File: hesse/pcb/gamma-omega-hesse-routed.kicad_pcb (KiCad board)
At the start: 2 copper layers, 232.8 x 111.4 mm, 47 parts

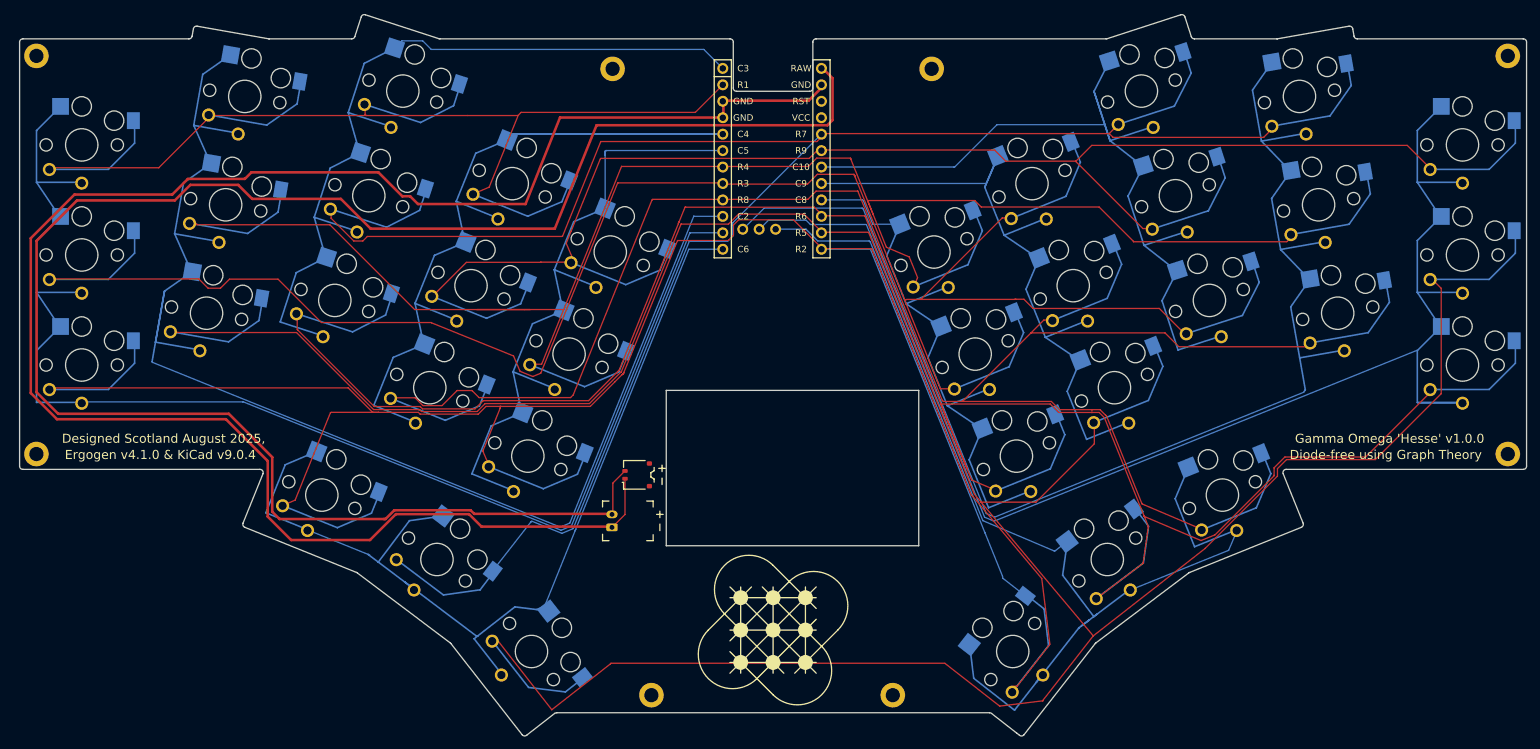
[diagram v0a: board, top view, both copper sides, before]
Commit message: clean
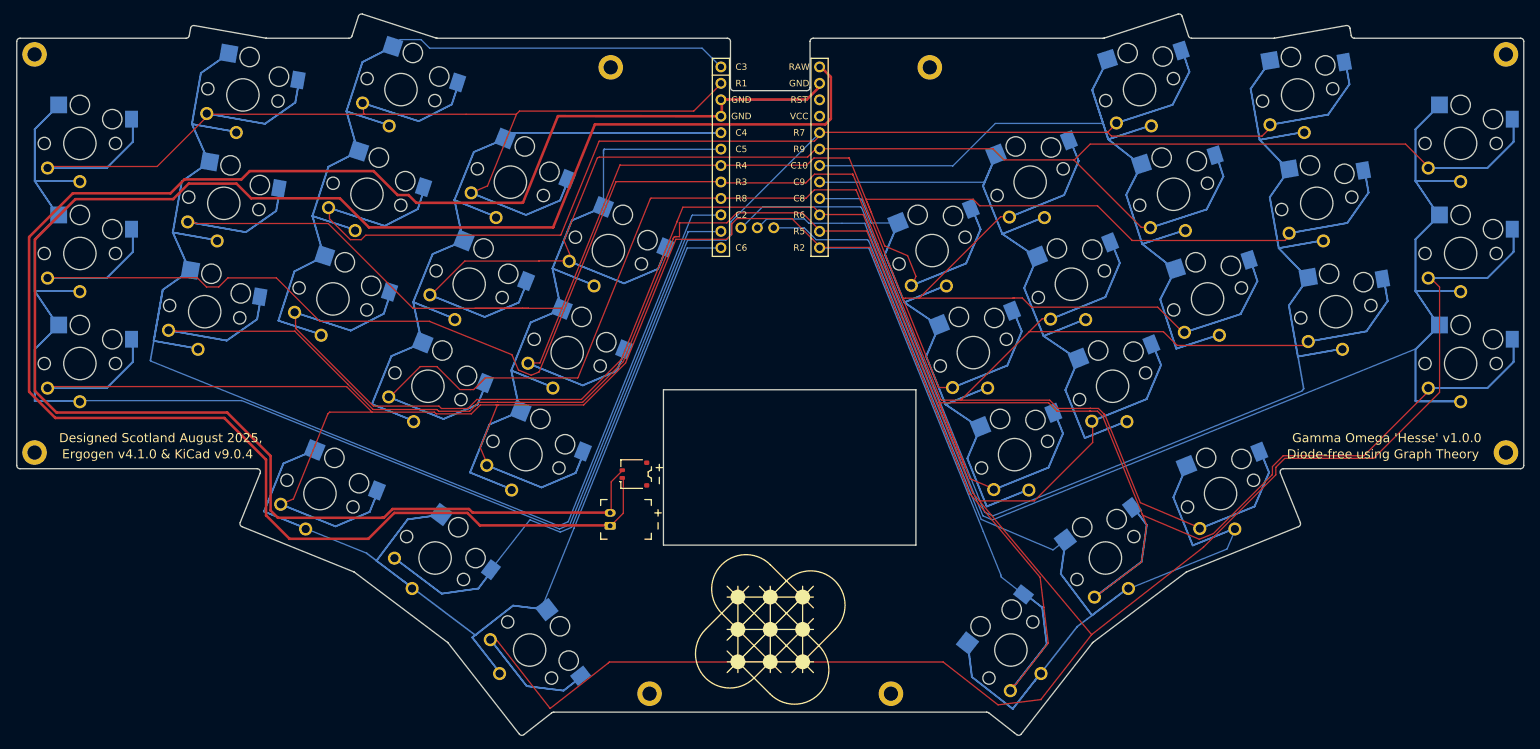
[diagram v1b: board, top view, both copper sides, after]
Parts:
- moved CONN1 0.43 mm to (135.2, 117.2)
- moved S24 0.37 mm to (237.6, 58.7)
- moved S4 0.37 mm to (68.8, 92.2)
- moved S6 0.37 mm to (74.7, 58.7)
- moved S12 0.37 mm to (116.0, 72.2)
- moved S31 0.37 mm to (193.9, 114.2)
- moved S10 0.37 mm to (103.3, 103.7)
- moved H6 0.37 mm to (180.8, 54.4)
- moved S8 0.37 mm to (93.9, 74.0)
- moved S9 0.37 mm to (99.1, 57.9)
- moved S15 0.37 mm to (131.2, 82.7)
- moved S5 0.37 mm to (71.7, 75.4)
- moved S23 0.37 mm to (240.6, 75.4)
- moved JST1 0.37 mm to (131.4, 124.2)
- moved S21 0.37 mm to (262.8, 66.2)
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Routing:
- net R5: track 495.9 -> 569.3 mm
- net R7: track 328.3 -> 401.3 mm
- net R1: track 198.1 -> 271.0 mm
- net R4: track 308.9 -> 381.7 mm
- net R9: track 259.0 -> 331.8 mm
- net R3: track 327.5 -> 400.2 mm
- net C1: track 205.6 -> 278.1 mm
- net C4: track 161.9 -> 234.3 mm
- net C3: track 124.0 -> 196.4 mm
- net C9: track 102.8 -> 175.2 mm
- net C5: track 100.3 -> 172.7 mm
- net C8: track 87.0 -> 159.4 mm
- net C12: track 217.6 -> 289.9 mm
- net C11: track 201.5 -> 273.8 mm
- net C10: track 126.9 -> 199.3 mm
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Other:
- outline, holes or cut-outs redrawn

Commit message: shift
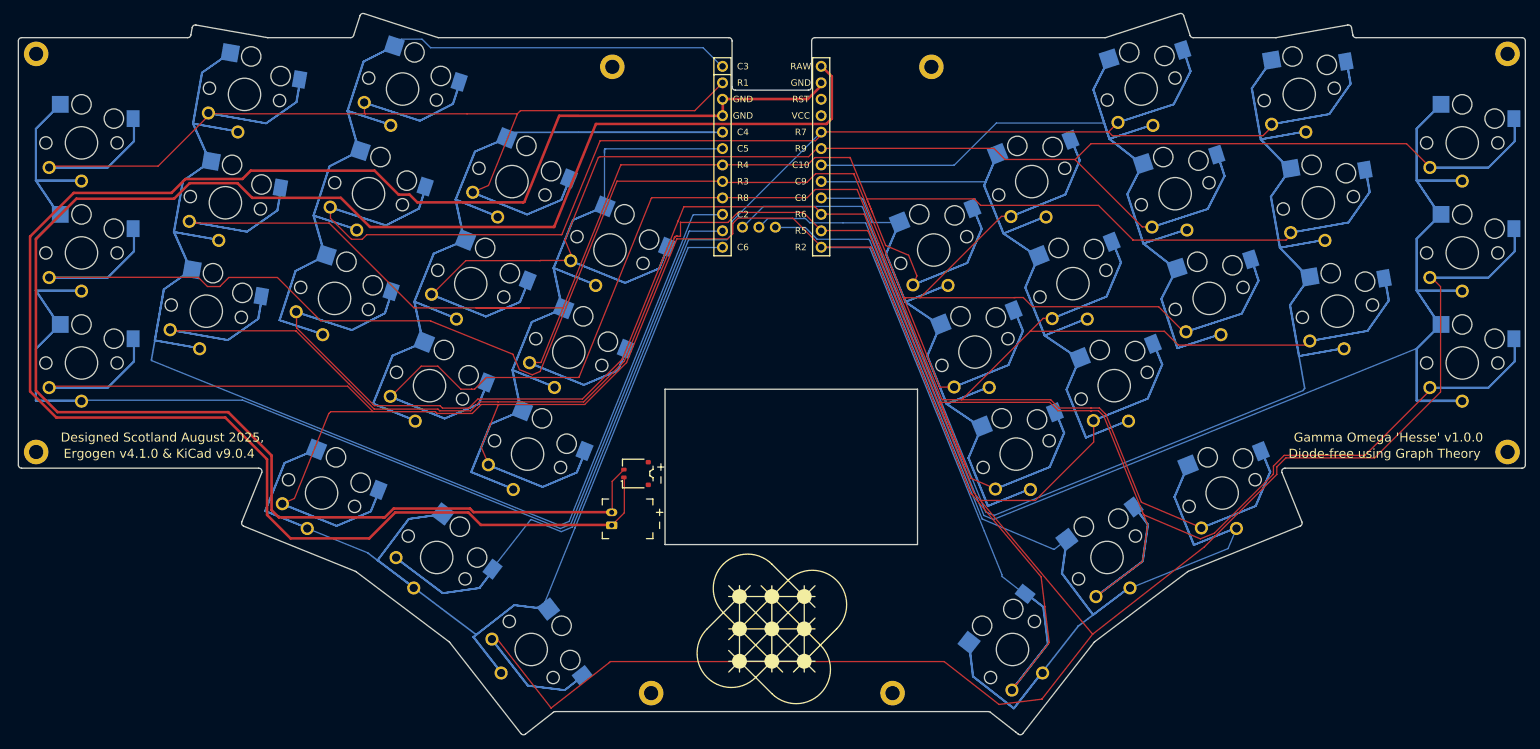
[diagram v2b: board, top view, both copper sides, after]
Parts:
- moved S14 0.26 mm to (125.0, 98.4)
- moved S5 0.26 mm to (72.0, 75.3)
- moved S2 0.26 mm to (49.8, 83.1)
- moved S12 0.26 mm to (116.3, 72.1)
- moved JST1 0.26 mm to (131.7, 124.2)
- moved S7 0.26 mm to (88.8, 90.1)
- moved S35 0.26 mm to (208.2, 130.1)
- moved S25 0.26 mm to (223.9, 90.1)
- moved H6 0.26 mm to (181.0, 54.3)
- moved H3 0.26 mm to (42.8, 113.8)
- moved S15 0.26 mm to (131.4, 82.6)
- moved S1 0.26 mm to (49.8, 100.1)
- moved H1 0.26 mm to (42.8, 52.3)
- moved S11 0.26 mm to (109.9, 87.8)
- moved S33 0.26 mm to (181.4, 82.6)
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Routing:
- net R7: track 401.3 -> 474.2 mm
- net R9: track 331.8 -> 404.8 mm
- net R3: track 400.2 -> 473.1 mm
- net R1: track 271.0 -> 343.9 mm
- net R8: track 390.5 -> 463.4 mm
- net R6: track 435.9 -> 508.8 mm
- net R2: track 471.0 -> 543.9 mm
- net R5: track 569.3 -> 642.2 mm
- net R4: track 381.7 -> 454.6 mm
- net C12: track 289.9 -> 362.3 mm
- net C9: track 175.2 -> 247.6 mm
- net C5: track 172.7 -> 245.0 mm
- net C1: track 278.1 -> 350.4 mm
- net C8: track 159.4 -> 231.8 mm
- net C2: track 281.1 -> 353.4 mm
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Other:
- outline, holes or cut-outs redrawn

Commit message: clean
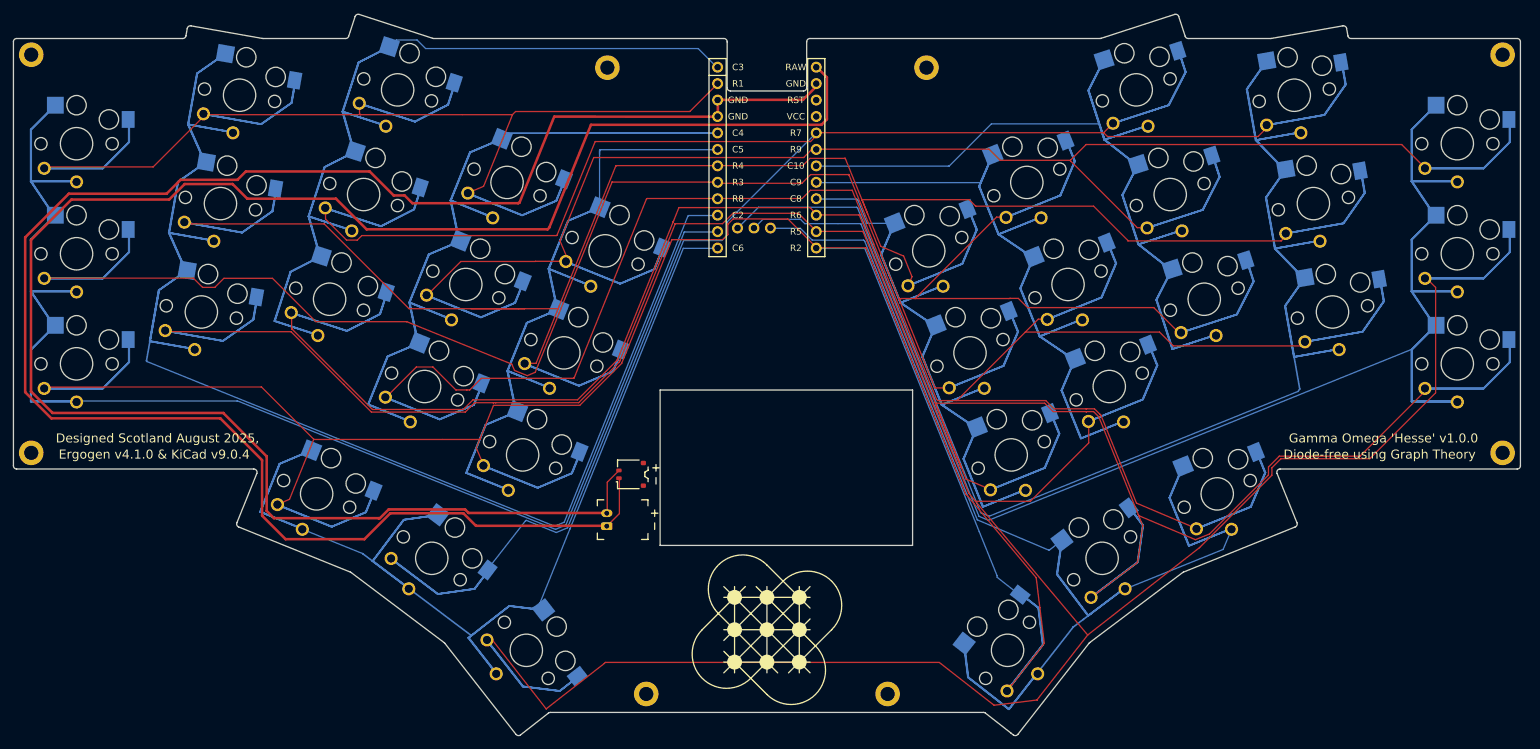
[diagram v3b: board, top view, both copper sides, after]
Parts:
- moved H1 0.77 mm to (42.0, 52.5)
- moved S15 0.77 mm to (130.6, 82.8)
- moved H6 0.77 mm to (180.3, 54.5)
- moved H5 0.77 mm to (131.0, 54.5)
- moved S14 0.77 mm to (124.3, 98.5)
- moved S1 0.77 mm to (49.0, 100.2)
- moved H2 0.77 mm to (269.3, 52.5)
- moved S7 0.77 mm to (88.1, 90.2)
- moved S6 0.77 mm to (74.2, 58.7)
- moved S12 0.77 mm to (115.5, 72.2)
- moved S21 0.77 mm to (262.3, 66.2)
- moved S5 0.77 mm to (71.2, 75.5)
- moved CONN1 0.77 mm to (134.6, 117.3)
- moved H4 0.77 mm to (269.3, 114.0)
- moved S27 0.77 mm to (212.7, 57.9)
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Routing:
- net R2: track 543.9 -> 531.7 mm
- net R5: track 642.2 -> 641.5 mm
- net R3: track 473.1 -> 472.4 mm
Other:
- outline, holes or cut-outs redrawn
